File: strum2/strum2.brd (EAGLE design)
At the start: 167.6 x 99.1 mm, 99 parts, among them IC1 REG1117, IC2 MCU-PIC16F1825-I/ST(TSSOP14), IC3 74HC595D, IC4 74HC595D, SW1 12MMTACT_SMT, SW10 12MMTACT_SMT, SW11 12MMTACT_SMT, SW12 12MMTACT_SMT, SW13 12MMTACT_SMT, SW14 12MMTACT_SMT, SW15 12MMTACT_SMT, SW16 12MMTACT_SMT, SW17 12MMTACT_SMT, SW18 12MMTACT_SMT, SW19 12MMTACT_SMT, SW2 12MMTACT_SMT, SW20 12MMTACT_SMT, SW21 12MMTACT_SMT, SW22 12MMTACT_SMT, SW23 12MMTACT_SMT, SW24 12MMTACT_SMT, SW25 12MMTACT_SMT, SW26 12MMTACT_SMT, SW27 12MMTACT_SMT, SW28 12MMTACT_SMT, SW29 12MMTACT_SMT, SW3 12MMTACT_SMT, SW30 12MMTACT_SMT, SW31 12MMTACT_SMT, SW32 12MMTACT_SMT, SW33 12MMTACT_SMT, SW34 12MMTACT_SMT, SW35 12MMTACT_SMT, SW36 12MMTACT_SMT, SW4 12MMTACT_SMT, SW5 12MMTACT_SMT, SW6 12MMTACT_SMT, SW7 12MMTACT_SMT, SW8 12MMTACT_SMT, SW9 12MMTACT_SMT

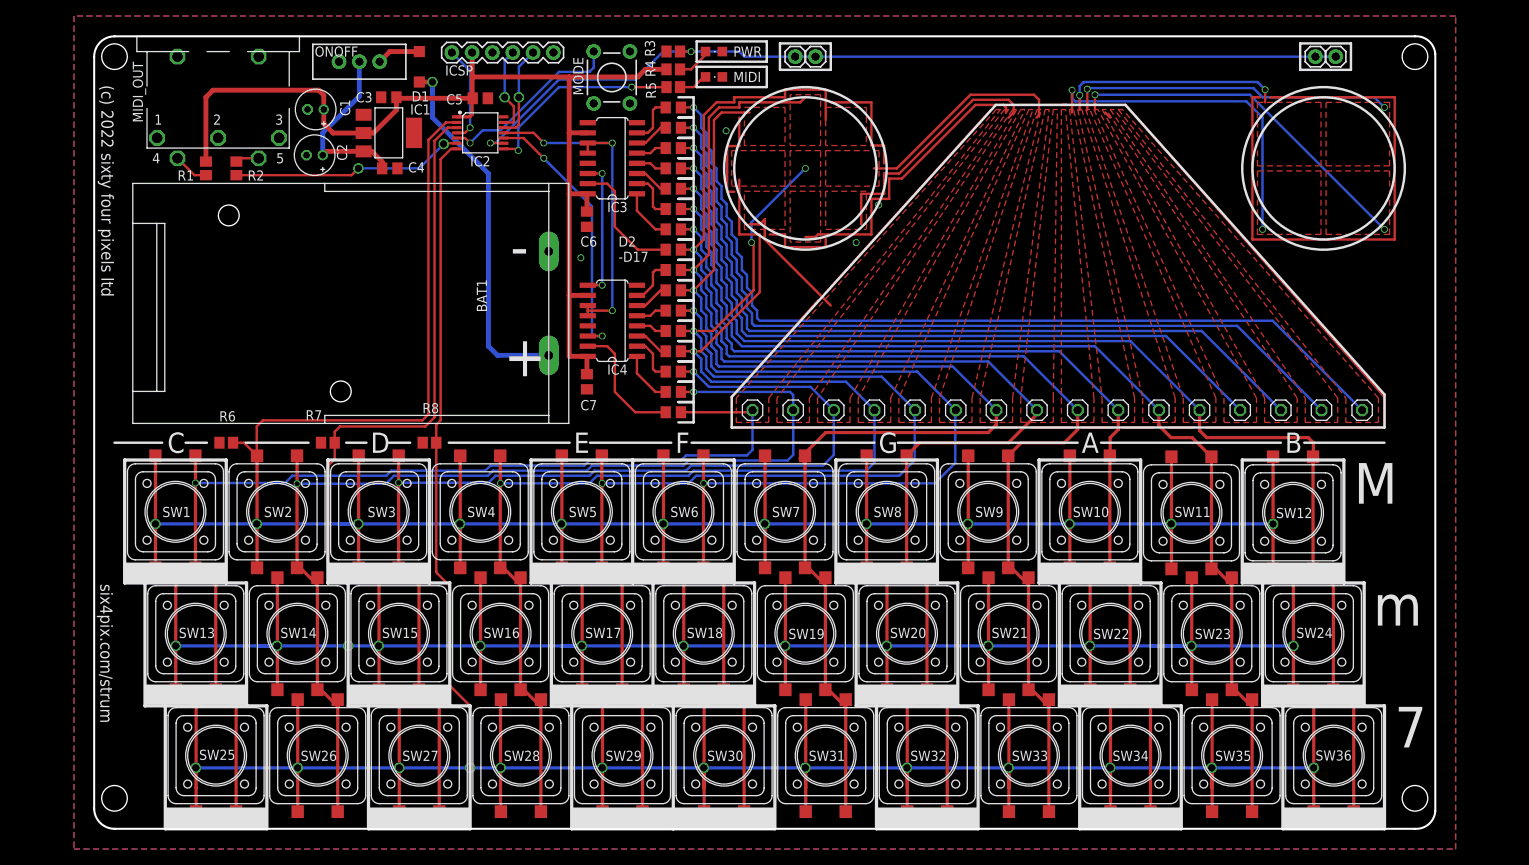
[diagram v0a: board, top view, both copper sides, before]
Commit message: asasas
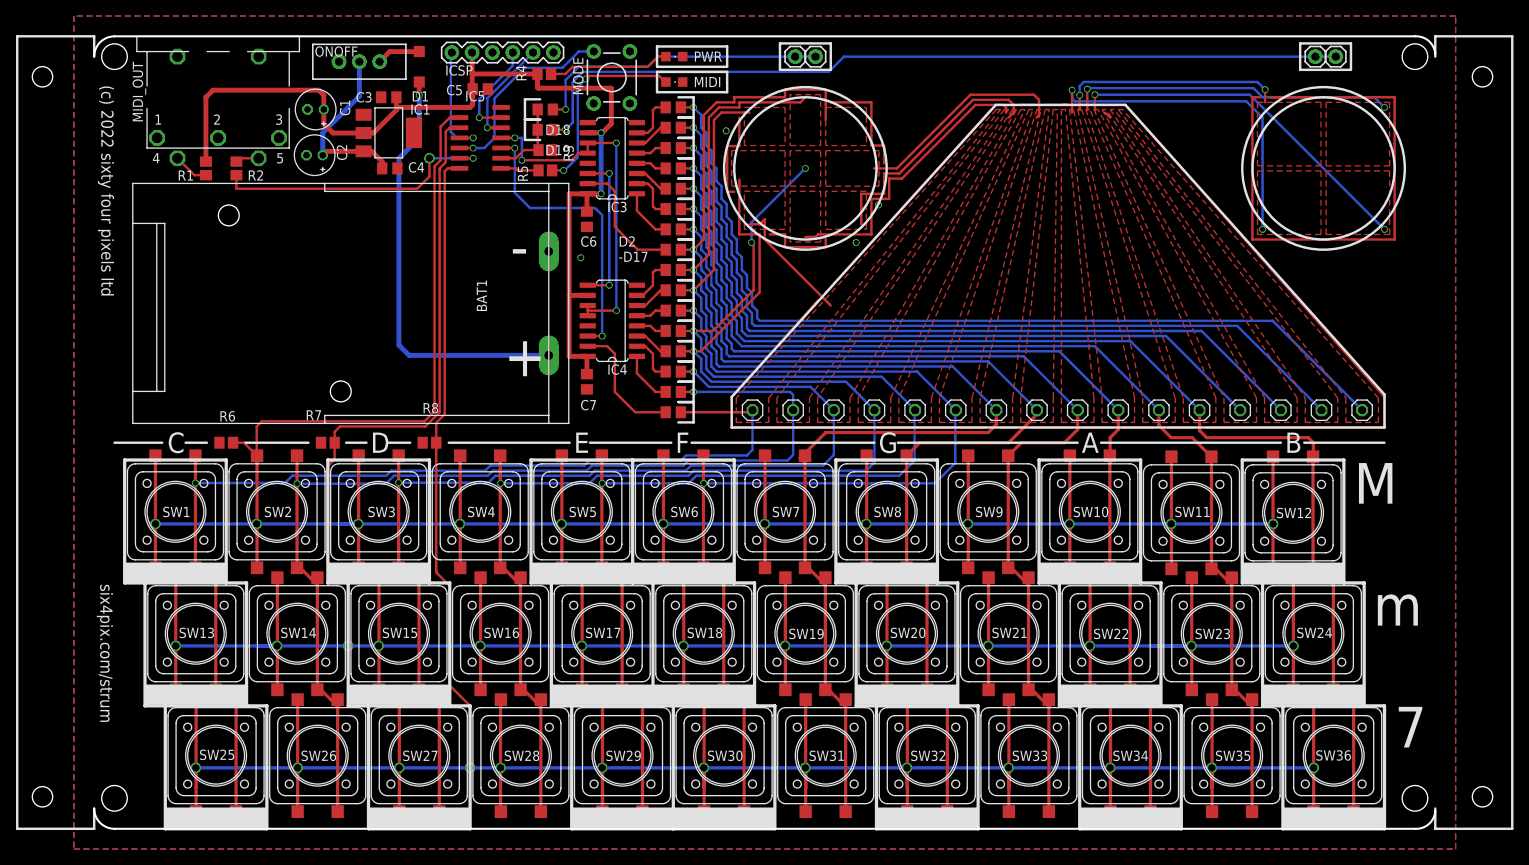
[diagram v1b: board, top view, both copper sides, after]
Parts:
- removed IC2: MCU-PIC16F1825-I/ST(TSSOP14), MCU-PIC16F1825-I_ST_TSSOP14_:TSSOP14-0.65-5X4.4MM
- added D18, D19: (no value), jason_eagle6:D0805
- added IC5: PIC16F1825SO14, jasons_stuff:SO14
- moved STYLUS 65.0 mm to (150.1, 96.5)
- moved STYLUS3 65.0 mm to (85.1, 96.5)
- moved R3 20.2 mm to (53.8, 84.8), turned to 180 degrees
- moved R5 19.1 mm to (53.8, 82.3)
- moved R4 16.1 mm to (53.7, 94.4)
- moved MIDI 4.99 mm to (70.0, 93.3)
- moved PWR 4.99 mm to (70.0, 96.5)
- moved C5 1.14 mm to (45.7, 92.5)
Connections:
- new net N$24: D18.A, STYLUS2.1, STYLUS3.1
- new net N$25: D19.A, STYLUS.1, STYLUS1.1
- net GND: now also IC5.14; no longer IC2.14
- net RA0: now also IC5.13; no longer IC2.13
- net RA1: now also IC5.12; no longer IC2.12
- net RA2: now also IC5.11; no longer IC2.11
- net RA3: now also IC5.4; no longer IC2.4
- net RA4: now also IC5.3; no longer IC2.3
- net RA5: now also IC5.2; no longer IC2.2
- net RC0: now also IC5.10; no longer IC2.10
- net RC1: now also D18.K, D19.K, IC5.9; no longer IC2.9, STYLUS.1, STYLUS1.1, STYLUS2.1, STYLUS3.1
- net RC2: now also IC5.8; no longer IC2.8
- net RC3: now also IC5.7; no longer IC2.7
- net RC4: now also IC5.6; no longer IC2.6
- net RC5: now also IC5.5; no longer IC2.5
- net VCC: now also IC5.1; no longer IC2.1
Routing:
- net N$25: track 0.00 -> 104.6 mm, vias 0 -> 1
- net RC1: track 113.7 -> 10.2 mm, vias 2 -> 0
- net N$24: track 0.00 -> 37.7 mm, vias 0 -> 1
- net N$12: track 3.71 -> 25.0 mm, vias 0 -> 2
- net RC2: track 25.4 -> 4.79 mm, vias 2 -> 0
- net N$1: track 4.34 -> 15.3 mm
- net VCC: track 132.2 -> 123.8 mm, vias 0 -> 2
- net N$2: track 45.6 -> 53.2 mm
- net RC4: track 29.2 -> 35.9 mm
- net RC0: track 33.7 -> 36.3 mm
- net RA3: track 12.3 -> 14.8 mm
- net RC3: track 408.4 -> 406.5 mm
- net CARRY: track 17.6 -> 19.4 mm
- net RA0: track 10.8 -> 12.6 mm
- net RA1: track 11.8 -> 13.5 mm
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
